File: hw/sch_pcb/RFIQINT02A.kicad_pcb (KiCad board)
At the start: 2 copper layers, 40.1 x 60.5 mm, 33 parts, among them J1 HEADER_2x03_PARALLEL, J2 HEADER_2x04_PARALLEL, J3 SATA7-67491-1030, J4 SATA7-67491-1030, J5 SATA7-67491-1030, J6 RJ45_RJHSE-5384, J7 RJ45_RJHSE-5384, M1 HOLE, M2 HOLE, M3 HOLE, M4 HOLE, U1 Si53322

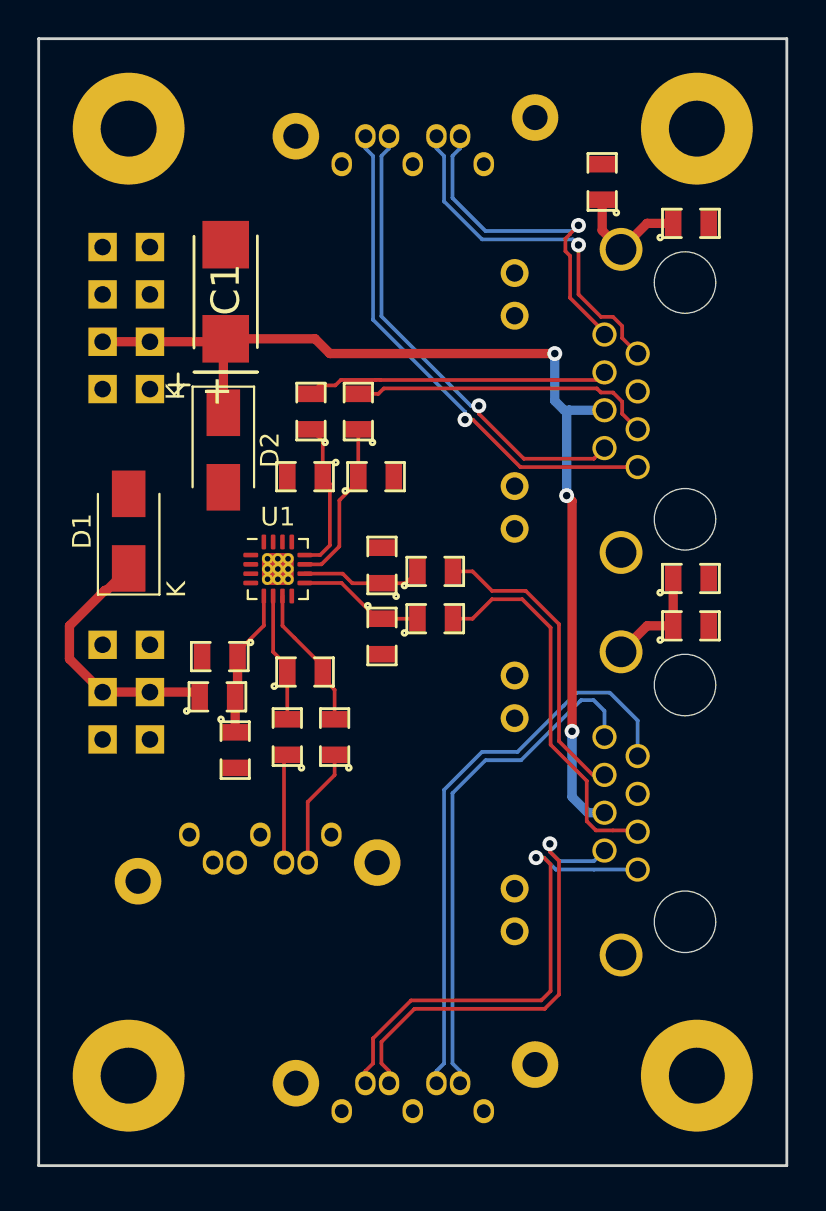
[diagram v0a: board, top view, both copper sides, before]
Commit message: Edit PCB
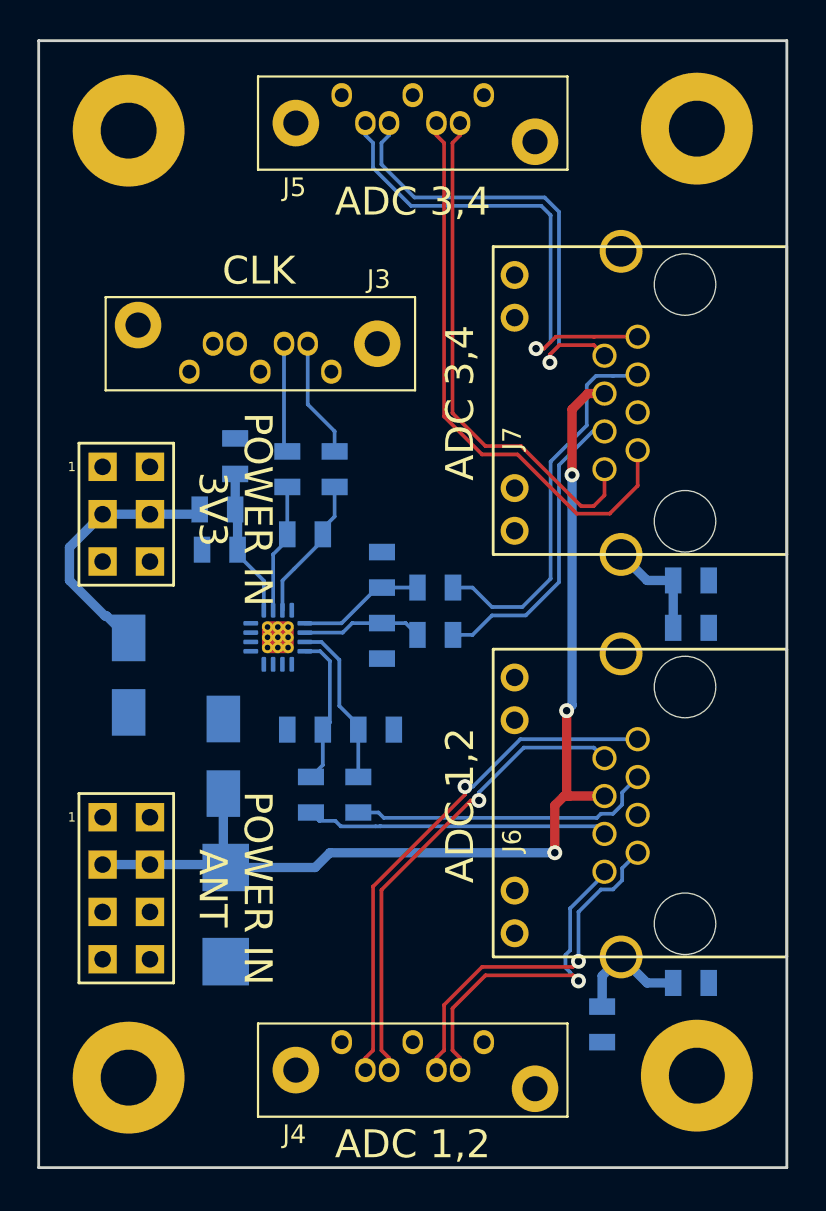
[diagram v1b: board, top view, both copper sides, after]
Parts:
- C1, C10, C11, C2, C3, C4, C5, C6, C7, C8, C9, D1, D2, L1, M2, M4, R1, R2, R3, R4, R5, R6, R7, U1: moved to B.Cu
- J1, J2, J3, J4, J5, J6, J7: moved to F.Cu
- moved M4 164.7 mm to (5.08, -55.8)
- moved J5 54.5 mm to (16.5, -57.7)
- moved M2 50.9 mm to (5.08, -4.97)
- moved J4 47.1 mm to (16.5, -6.88)
- moved C10 45.2 mm to (30.5, -7.83), turned to -90 degrees
- moved R6 40.7 mm to (35.2, -10.1)
- moved J6 34.4 mm to (34.9, -13.2), turned to 90 degrees
- moved C1 33.4 mm to (10.3, -13.7), turned to -90 degrees
- moved J2 30.6 mm to (4.95, -15.1)
- moved J3 24.8 mm to (16.0, -42.8)
- moved C8 20.6 mm to (17.4, -20.1), turned to -90 degrees
- moved C9 20.6 mm to (14.9, -20.1), turned to -90 degrees
- moved D2 16.4 mm to (10.2, -22.2), turned to 90 degrees
- moved C2 15.8 mm to (10.8, -38.3), turned to 90 degrees
- moved C3 14.4 mm to (13.6, -37.6), turned to -90 degrees
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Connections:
- M4 pad 1: Net-(M4-Pad1) -> GND
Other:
- board text added: "ADC 1,2"
- board text added: "ADC 3,4"
- board text added: "CLK"
- board text added: "POWER IN 3V3"
- board text added: "POWER IN ANT"
